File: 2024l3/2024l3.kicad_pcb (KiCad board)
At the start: 2 copper layers, 133 x 90.5 mm, 39 parts, among them J1 Conn_01x06, J2 TOF 0, J3 TOF 1, J4 TOF 2, J5 TOF 3, SW1 SW_SPDT, SW2 SW_SPDT, SW3 SW_SPDT, SW4 SW_SPDT, SW5 SW_SPDT, SW6 SW_SPDT, U1 OpenMV, U2 4754, U3 >VALUE, U4 Adafruit Featherwing, U5 Teensy 4.0, U6 >VALUE

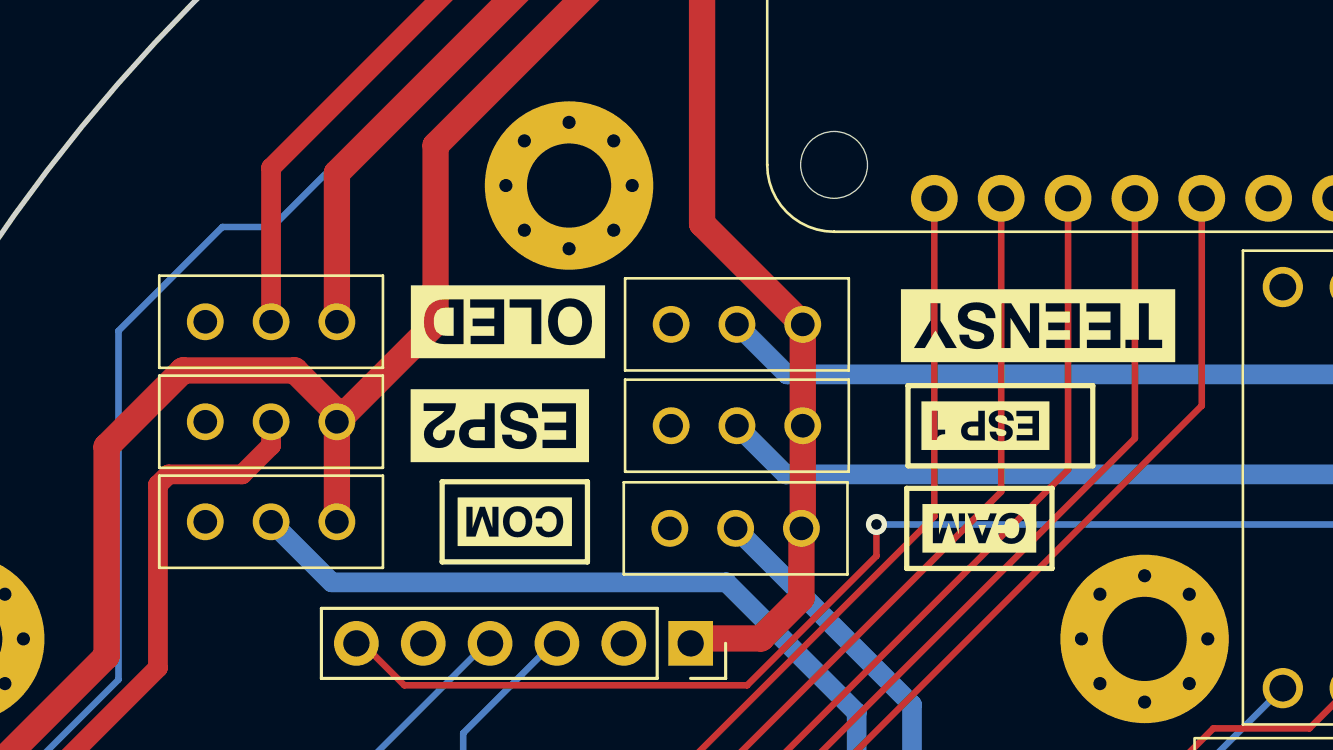
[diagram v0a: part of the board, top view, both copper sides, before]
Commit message: L3 Silk
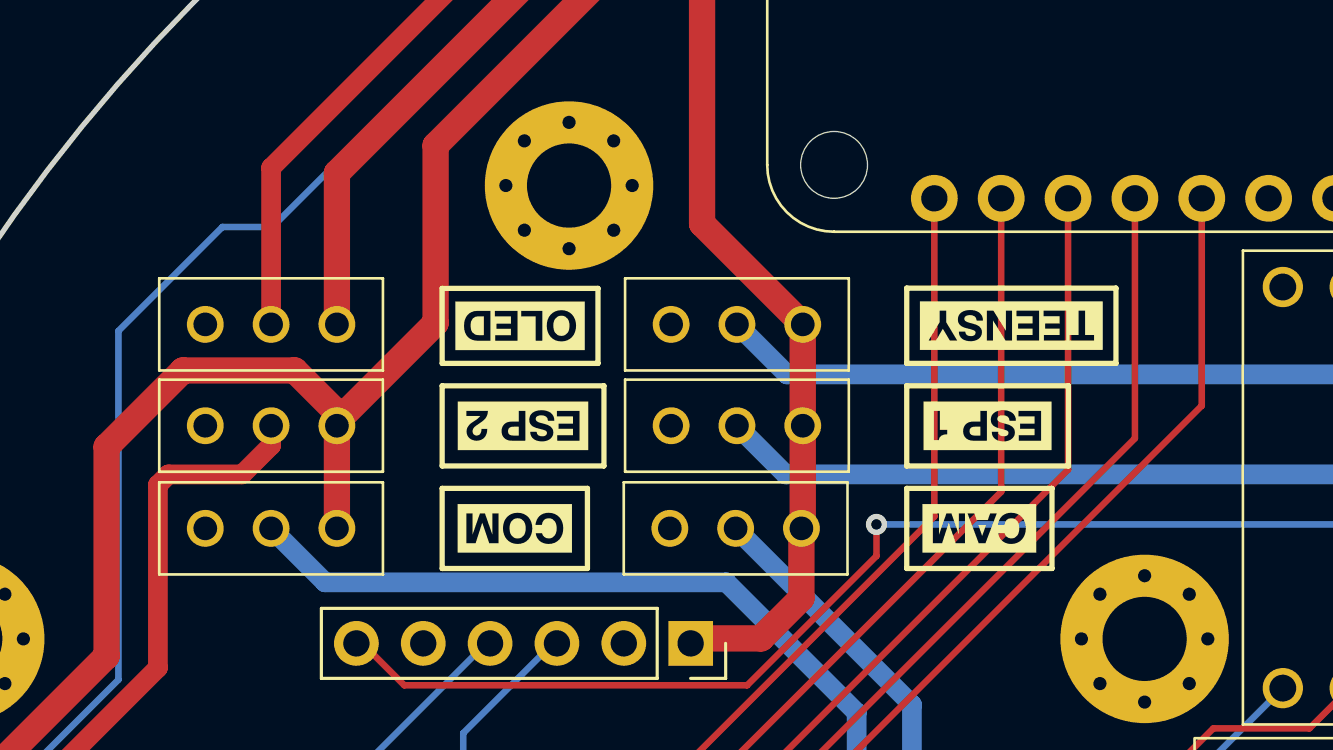
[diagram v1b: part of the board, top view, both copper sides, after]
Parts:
- removed kibuzzard-65630B66: G***, kibuzzard-65630B66
- removed kibuzzard-657BF16E: G***, kibuzzard-657BF16E
- removed kibuzzard-657BF185: G***, kibuzzard-657BF185
- added kibuzzard-659111B0: G***, kibuzzard-659111B0, F.Cu at (113.9, 70.3)
- added kibuzzard-659111BA: G***, kibuzzard-659111BA, F.Cu at (132.6, 70.3)
- added kibuzzard-65911205: G***, kibuzzard-65911205, F.Cu at (114.0, 74.1)
- moved kibuzzard-6590F814 0.25 mm to (113.7, 78.0)
- moved SW1 0.25 mm to (104.4, 78.0)
- moved SW6 0.15 mm to (104.4, 74.1)
- moved SW3 0.10 mm to (104.4, 70.3)
- moved kibuzzard-6590F77B 0.08 mm to (131.7, 74.1)

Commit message: LCSC Updates
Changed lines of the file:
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@@
     (attr board_only exclude_from_pos_files exclude_from_bom)
     (fp_text reference "kibuzzard-65911205" (at 0 -3.97166 180) (layer "F.SilkS") hide
-        (effects (font (size 0 0)))
+        (effects (font (size 0 0) (thickness 0.15)))
     )
     (fp_text value "G***" (at 0 3.97166 180) (layer "F.SilkS") hide
-        (effects (font (size 0 0)))
+        (effects (font (size 0 0) (thickness 0.15)))
     )
     (fp_poly
@@
     (attr board_only exclude_from_pos_files exclude_from_bom)
     (fp_text reference "kibuzzard-659111BA" (at 0 -3.97166 180) (layer "F.SilkS") hide
-        (effects (font (size 0 0)))
+        (effects (font (size 0 0) (thickness 0.15)))
     )
     (fp_text value "G***" (at 0 3.97166 180) (layer "F.SilkS") hide
-        (effects (font (size 0 0)))
+        (effects (font (size 0 0) (thickness 0.15)))
     )
     (fp_poly
@@
     (attr board_only exclude_from_pos_files exclude_from_bom)
     (fp_text reference "kibuzzard-659111B0" (at 0 -3.97166 180) (layer "F.SilkS") hide
-        (effects (font (size 0 0)))
+        (effects (font (size 0 0) (thickness 0.15)))
     )
     (fp_text value "G***" (at 0 3.97166 180) (layer "F.SilkS") hide
-        (effects (font (size 0 0)))
+        (effects (font (size 0 0) (thickness 0.15)))
     )
     (fp_poly
@@
     )
   )
-  (gr_rect (start 128.585 71.77) (end 136.535 68.91)
+  (gr_rect (start 128.585 68.91) (end 136.535 71.77)
     (stroke (width 0.2) (type default)) (fill none) (layer "F.SilkS"))
   (gr_rect (start 128.585 72.6215) (end 134.73 75.6665)
@@
   (gr_rect (start 110.935 72.6215) (end 117.08 75.6665)
     (stroke (width 0.2) (type default)) (fill none) (layer "F.SilkS"))
-  (gr_rect (start 110.935 71.77) (end 116.855 68.92)
+  (gr_rect (start 110.935 68.92) (end 116.855 71.77)
     (stroke (width 0.2) (type default)) (fill none) (layer "F.SilkS"))
   (gr_rect (start 128.585 76.518) (end 134.105 79.563)
